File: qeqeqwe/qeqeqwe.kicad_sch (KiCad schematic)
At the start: 10 parts, among them J1 USB_A, J2 USB_A, U1 ATtiny85-20S

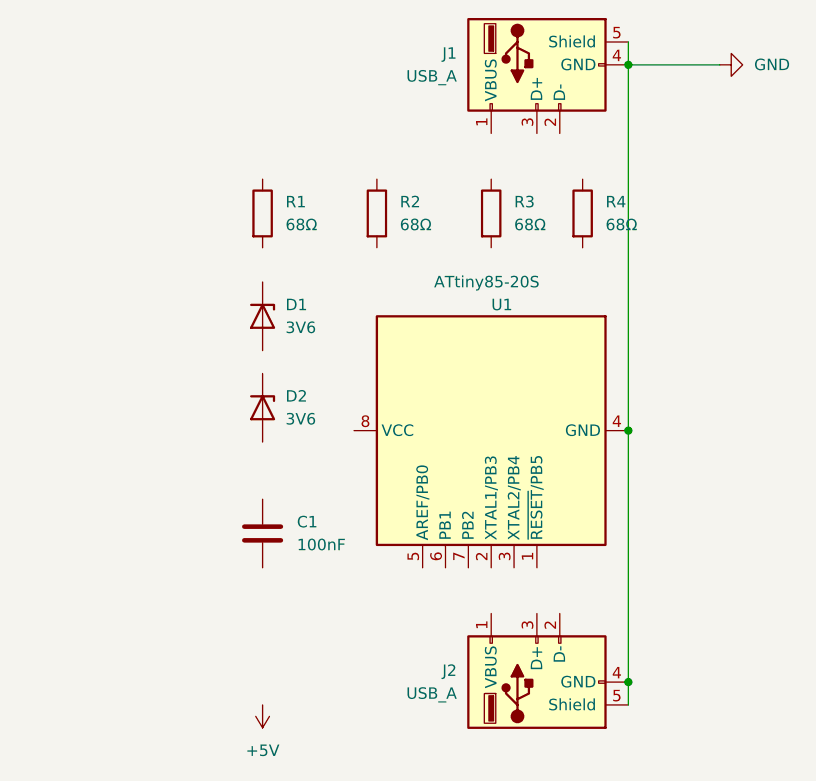
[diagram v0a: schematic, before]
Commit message: we
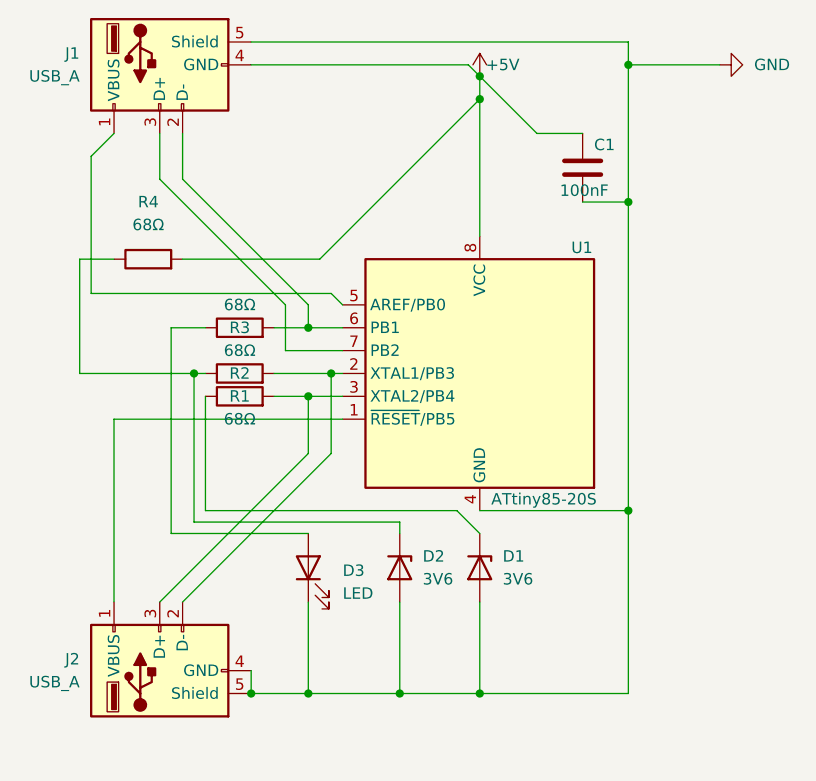
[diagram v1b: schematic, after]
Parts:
- added D3: LED, LED_THT:LED_D5.0mm, symbol Device:LED
- J1, J2: footprint (none) -> Connector_USB:USB_A_Receptacle_GCT_USB1046
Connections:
- net +5V: now also C1.1, J1.4 (GND), R4.2, U1.8 (VCC)
- net GND: now also C1.2, D1.2 (A), D2.2 (A), D3.1 (K); no longer J1.4 (GND)
- net at U1.1 (~{RESET}/PB5): now also J2.1 (VBUS)
- net at U1.2 (XTAL1/PB3): now also J2.2 (D-), R2.2
- net at U1.3 (XTAL2/PB4): now also J2.3 (D+), R1.2
- net at U1.5 (AREF/PB0): now also J1.1 (VBUS)
- net at U1.6 (PB1): now also J1.2 (D-), R3.2
- net at U1.7 (PB2): now also J1.3 (D+)
- net at R4.1: now also D2.1 (K), R2.1
- net at R3.1: now also D3.2 (A)
- net at D1.1 (K): now also R1.1
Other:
- moved on the sheet: C1, D1, D2, J1, J2, R1, R2, R3, R4, U1
